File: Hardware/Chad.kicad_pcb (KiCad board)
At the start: 4 copper layers, 30 x 60 mm, 130 parts, among them J101 Conn_01x02_Male, J102 Conn_01x02_Male, J103 RBUS, J301 USB_C_Receptacle_USB2.0, J601 ServoCH0, J602 ServoCH1, J701 GPIO Breakout, Q501 SSM3K15AMFV,L3F, U101 ESP32-S3, U201 SN65HVD230, U401 LM66200DRLR, U402 MAX77827AEFD+T, U403 SC4215ASTRT, U501 SiC437AED-T1, Y101 R940000171

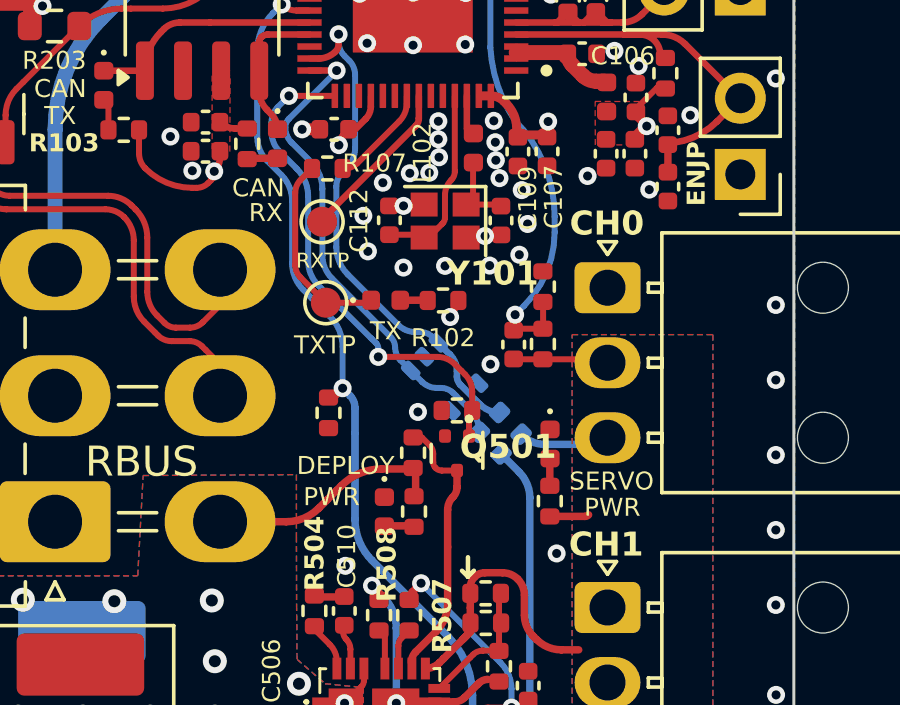
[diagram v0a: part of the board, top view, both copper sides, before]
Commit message: continued
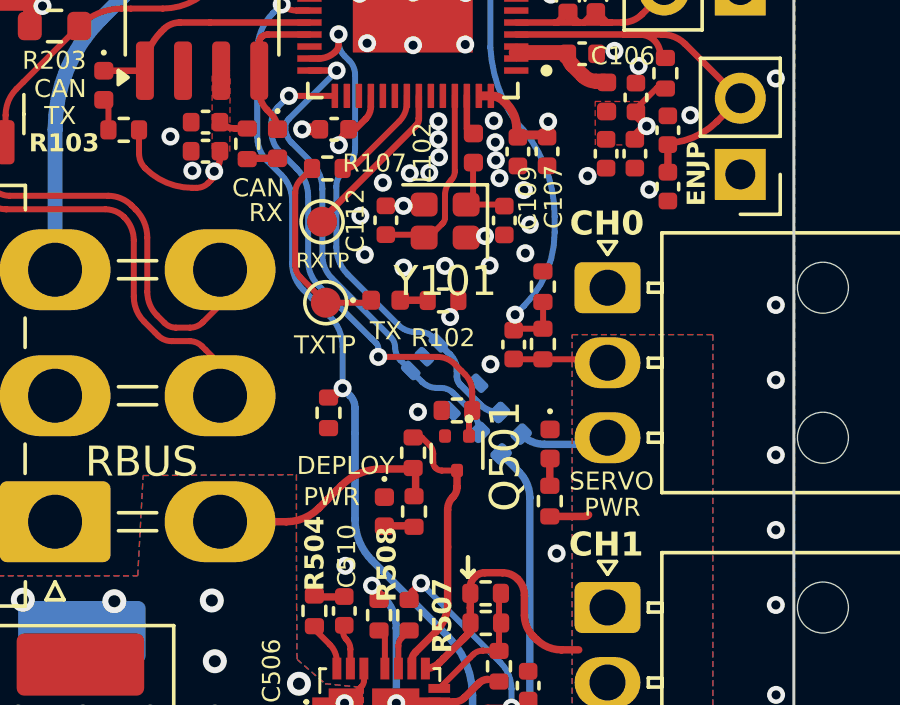
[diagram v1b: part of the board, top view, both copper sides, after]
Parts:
- D601: value ~ -> CPDV5-3V3UP-HF
- L101: value 2.0nH -> 2nH
- Q501: footprint iclr:SOT-723 -> Package_TO_SOT_SMD:SOT-723
- R101, R105: value 10K -> 10kΩ
- R102, R106, R111: value 470 -> 470Ω
- R103, R104, R109, R505: value 1k -> 1kΩ
- R107: value 499 -> 499Ω
- R108: value 3k -> 3kΩ
- R110: value 1.5k -> 1.5kΩ
- R112: value 18k -> 18kΩ
- R201: value 0 -> 0Ω
- R202, R203: value 60 -> 60Ω
- R301, R302, R303: value 5.1k -> 5.1kΩ
- R401, R404, R501, R503, R509, R701, R702, R703, R704, R705, R706: value 10k -> 10kΩ
- R402: value 14k -> 14kΩ
- R403: value 56k -> 56kΩ
- R502: value 113k -> 113kΩ
- R504: value 2.2 -> 2.2Ω
- R506: value 442k -> 442kΩ
- R507: value 200k -> 200kΩ
- R508: value 100k -> 100kΩ
- R510: value 5.1R -> 5.1Ω
- R601, R602: value 165R -> 165Ω
- U501: value SiC437AED-T1 -> SIC437AED-T1-GE3
- Y101: value R940000171 -> 40MHz±10ppm; footprint iclr:Crystal_SMD_2016-4Pin_2.0x1.6mm -> Crystal:Crystal_SMD_2016-4Pin_2.0x1.6mm
- moved C112 0.12 mm to (48.4, 68.8)
- moved C113 0.11 mm to (52.4, 68.8)
